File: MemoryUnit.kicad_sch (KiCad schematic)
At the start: 21 parts, among them U20 CY62256-70PC, U21 74LS30, U22 74LS32, U49 74LS377, U50 74LS30, U51 74LS138, U52 74LS377, U53 74LS377, U54 74HC541, U55 74HC541, U56 74LS377

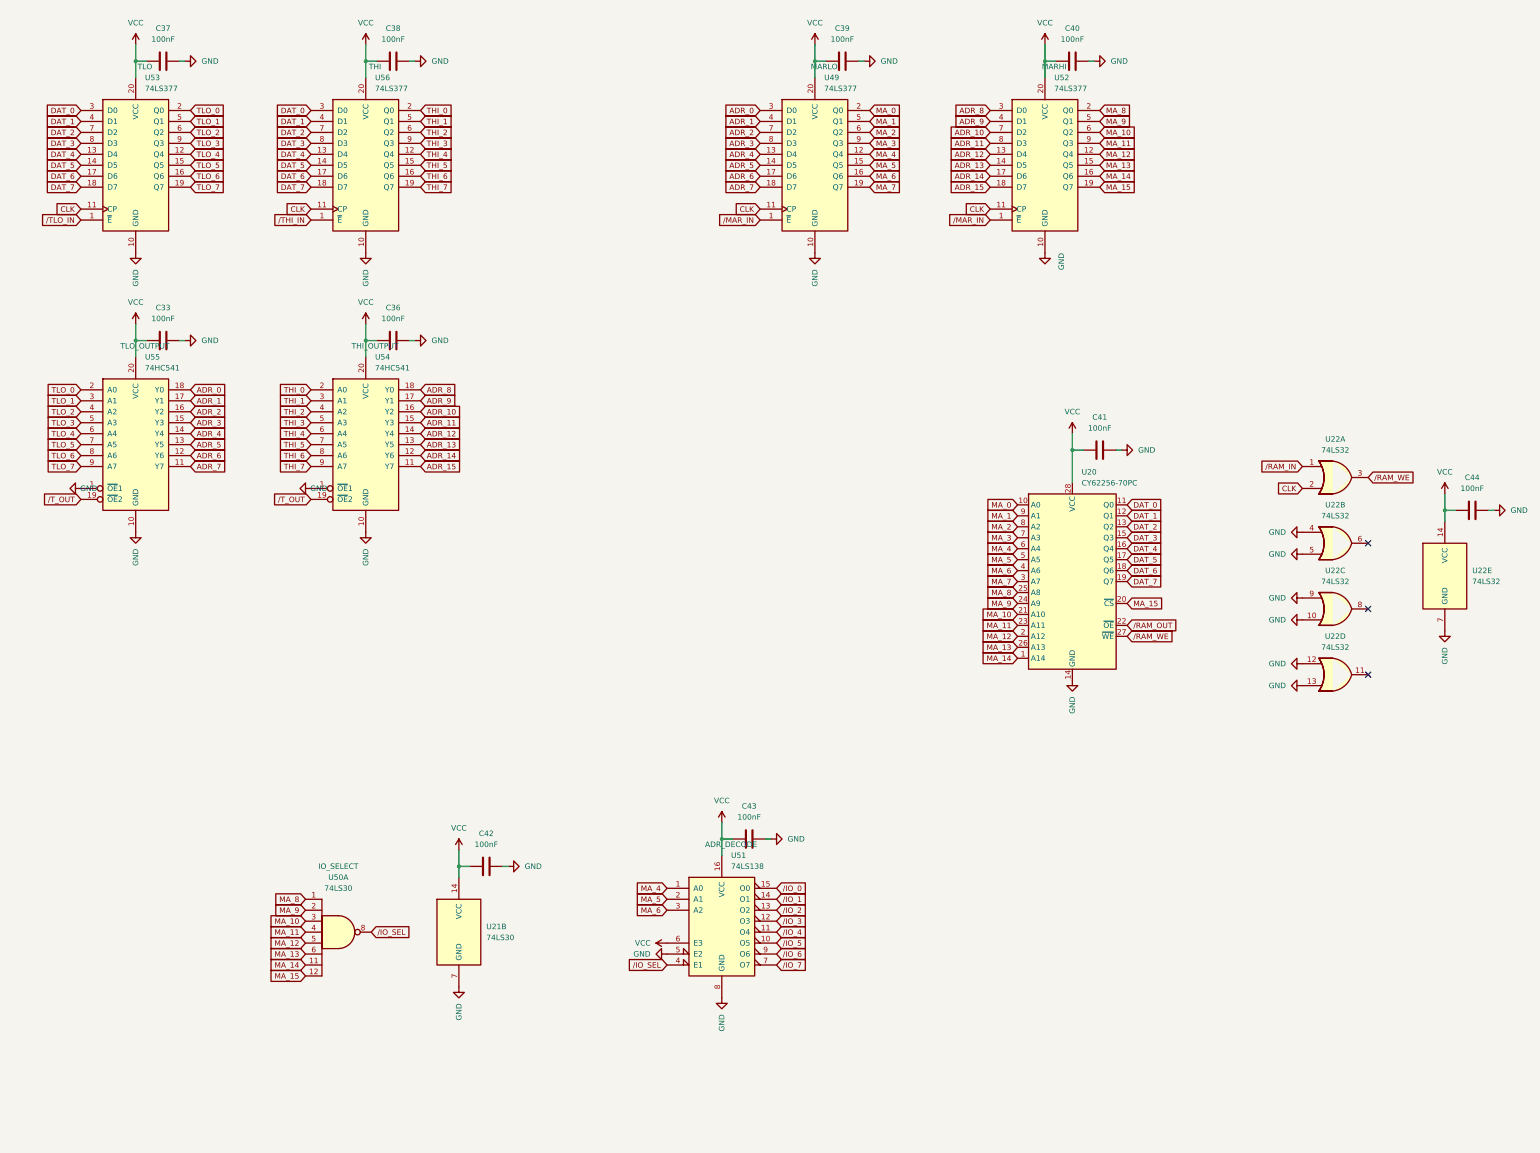
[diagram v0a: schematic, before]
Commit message: Fixes Gate symbol refs and adds backplane definition
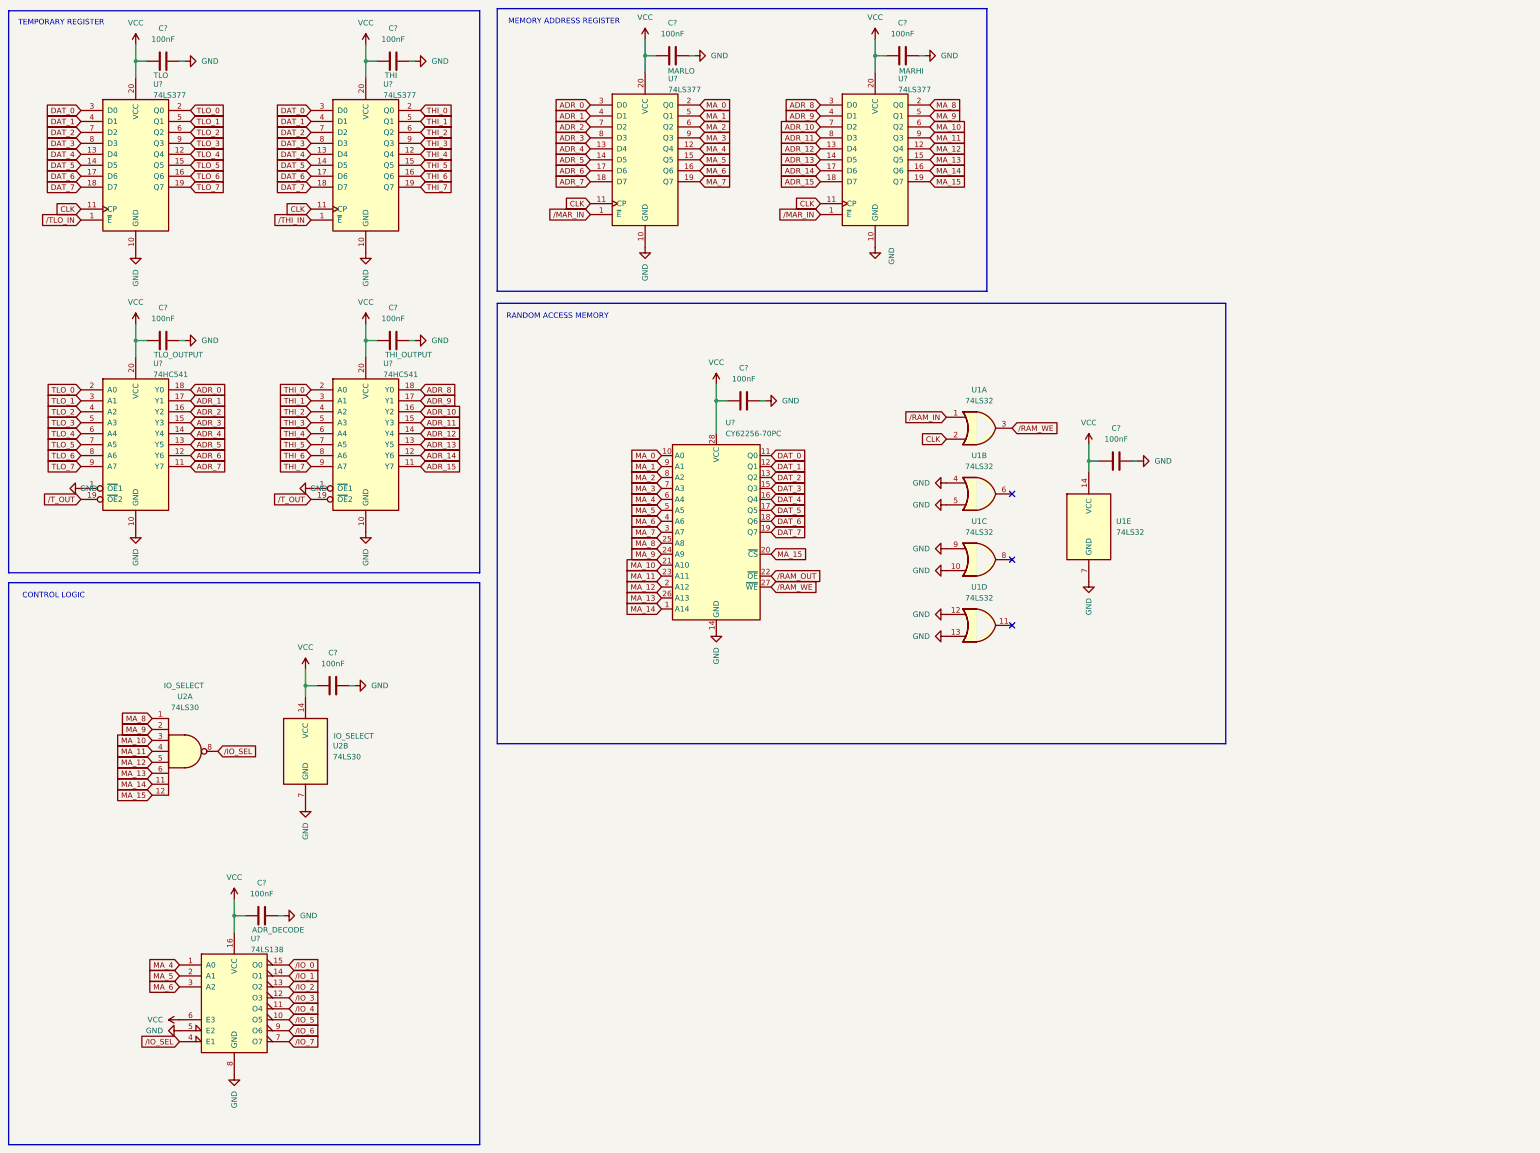
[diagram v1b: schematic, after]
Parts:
- removed U21, U50: 74LS30, Package_DIP:DIP-14_W7.62mm, symbol 74xx:74LS30
- removed U22: 74LS32, Package_DIP:DIP-14_W7.62mm, symbol 74xx:74LS32
- added U1: 74LS32, symbol 74xx:74LS32
- added U2: 74LS30, symbol 74xx:74LS30
- renumbered C36 to C?, C43 to C?, C33 to C?, C39 to C?, C37 to C?, C42 to C?, C44 to C?, C38 to C?, C41 to C?, C40 to C?, U49 to U?, U51 to U?, U20 to U?, U52 to U?, U53 to U?, U54 to U?, U55 to U?, U56 to U?
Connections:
- net CLK: now also U1.2
- net GND: now also U1.10, U1.12, U1.13, U1.4, U1.5, U1.7 (GND), U1.9, U2.7 (GND)
- net MA_10: now also U2.3
- net MA_11: now also U2.4
- net MA_12: now also U2.5
- net MA_13: now also U2.6
- net MA_14: now also U2.11
- net MA_15: now also U2.12
- net MA_8: now also U2.1
- net MA_9: now also U2.2
- net VCC: now also U1.14 (VCC), U2.14 (VCC)
- net /IO_SEL: now also U2.8
- net /RAM_IN: now also U1.1
- net /RAM_WE: now also U1.3
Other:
- note added: "CONTROL LOGIC"
- note added: "MEMORY ADDRESS REGISTER"
- note added: "RANDOM ACCESS MEMORY"
- note added: "TEMPORARY REGISTER"
- moved on the sheet: C?, U?
